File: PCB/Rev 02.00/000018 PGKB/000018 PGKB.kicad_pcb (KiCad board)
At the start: 4 copper layers, 93.5 x 72.5 mm, 154 parts, among them J1 USB Mini B, J2 BM04B-SRSS-TB, U1 SN74HCS365PWR, U2 SN74HCS365PWR, U3 SN74HCS365PWR, U4 W25Q80DVSSIG, U5 RP2040, U6 MCP1825T-3302E/DC, U7 CAT811TTBI-GT3, Y1 12 MHz

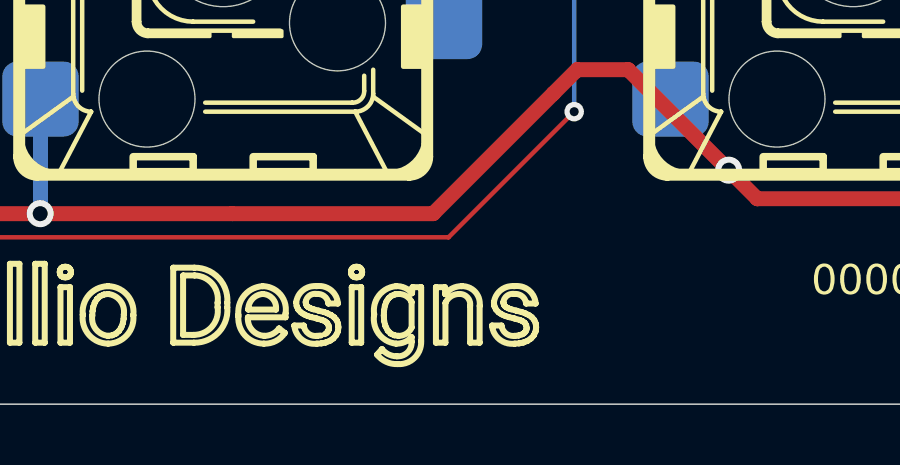
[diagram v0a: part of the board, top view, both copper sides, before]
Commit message: mfg files
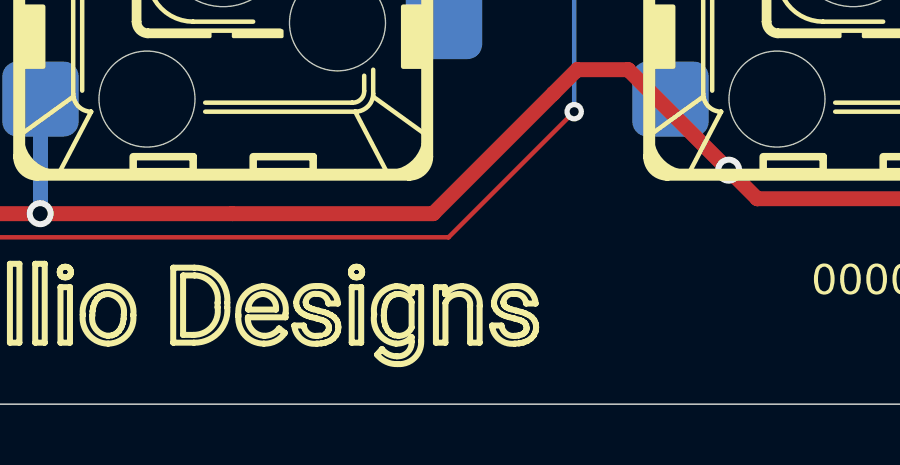
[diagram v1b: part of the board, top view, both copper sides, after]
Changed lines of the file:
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@@
     (fp_arc (start 0.833601 0.096099) (mid 0.973613 -0.257639) (end 1.31605 -0.423381)
       (stroke (width 0.2) (type solid)) (layer "F.SilkS"))
-    (fp_arc (start 1.31605 -0.683114) (mid 1.907699 -0.405492) (end 2.078018 0.225468)
+    (fp_arc (start 1.31605 -0.683114) (mid 1.907695 -0.405492) (end 2.078018 0.225468)
       (stroke (width 0.2) (type solid)) (layer "F.SilkS"))
     (fp_arc (start 1.31605 -0.423379) (mid 1.645394 -0.271037) (end 1.761468 0.072768)
@@
     (fp_arc (start 1.355618 1.232463) (mid 0.731987 0.965619) (end 0.50639 0.325909)
       (stroke (width 0.2) (type solid)) (layer "F.SilkS"))
-    (fp_arc (start 1.372869 0.972724) (mid 0.966364 0.781549) (end 0.82295 0.35584)
+    (fp_arc (start 1.372869 0.972724) (mid 0.966366 0.781547) (end 0.82295 0.35584)
       (stroke (width 0.2) (type solid)) (layer "F.SilkS"))
     (fp_arc (start 1.8609 0.725158) (mid 1.647116 0.90854) (end 1.372868 0.972731)
@@
     (fp_arc (start 3.12764 0.972723) (mid 2.834729 0.892832) (end 2.685781 0.628268)
       (stroke (width 0.2) (type solid)) (layer "F.SilkS"))
-    (fp_arc (start 3.12764 1.232463) (mid 2.619347 1.092399) (end 2.369218 0.628268)
+    (fp_arc (start 3.12764 1.232463) (mid 2.61934 1.092397) (end 2.369218 0.628268)
       (stroke (width 0.2) (type solid)) (layer "F.SilkS"))
-    (fp_arc (start 5.03409 0.259459) (mid 5.19195 -0.37288) (end 5.765118 -0.683118)
+    (fp_arc (start 5.03409 0.259459) (mid 5.191951 -0.372877) (end 5.765118 -0.683118)
       (stroke (width 0.2) (type solid)) (layer "F.SilkS"))
     (fp_arc (start 5.761569 1.232466) (mid 5.184943 0.905126) (end 5.03409 0.259459)
@@
     (fp_arc (start 5.844259 -0.423382) (mid 6.101988 -0.353589) (end 6.28105 -0.155518)
       (stroke (width 0.2) (type solid)) (layer "F.SilkS"))
-    (fp_arc (start 6.280538 1.013814) (mid 6.045436 1.181008) (end 5.761568 1.232468)
+    (fp_arc (start 6.280538 1.013814) (mid 6.045436 1.181019) (end 5.761568 1.232468)
       (stroke (width 0.2) (type solid)) (layer "F.SilkS"))
     (fp_arc (start 6.280541 1.169557) (mid 6.145913 1.523237) (end 5.79099 1.65455)
@@
     (fp_arc (start 7.400665 -0.416784) (mid 7.646446 -0.616044) (end 7.955659 -0.683118)
       (stroke (width 0.2) (type solid)) (layer "F.SilkS"))
-    (fp_arc (start 7.407765 -0.124568) (mid 7.589656 -0.340694) (end 7.859781 -0.423381)
+    (fp_arc (start 7.407765 -0.124568) (mid 7.589655 -0.340729) (end 7.859781 -0.423381)
       (stroke (width 0.2) (type solid)) (layer "F.SilkS"))
     (fp_arc (start 7.859779 -0.42338) (mid 8.138248 -0.314437) (end 8.231131 -0.030218)
       (stroke (width 0.2) (type solid)) (layer "F.SilkS"))
-    (fp_arc (start 7.955657 -0.683113) (mid 8.404847 -0.489303) (end 8.54819 -0.02159)
+    (fp_arc (start 7.955657 -0.683113) (mid 8.404805 -0.489301) (end 8.54819 -0.02159)
       (stroke (width 0.2) (type solid)) (layer "F.SilkS"))
     (fp_arc (start 9.023535 -0.141819) (mid 9.255576 -0.552139) (end 9.7084 -0.683118)
@@
     (fp_arc (start 9.708398 -0.683125) (mid 10.188203 -0.5481) (end 10.415081 -0.104281)
       (stroke (width 0.2) (type solid)) (layer "F.SilkS"))
-    (fp_arc (start 9.708398 -0.423378) (mid 9.96879 -0.344297) (end 10.097 -0.104281)
+    (fp_arc (start 9.708398 -0.423378) (mid 9.968762 -0.344292) (end 10.097 -0.104281)
       (stroke (width 0.2) (type solid)) (layer "F.SilkS"))
     (fp_arc (start 9.71855 0.972726) (mid 9.425639 0.892824) (end 9.276681 0.628268)
       (stroke (width 0.2) (type solid)) (layer "F.SilkS"))
-    (fp_arc (start 9.71855 1.232464) (mid 9.21027 1.092398) (end 8.960131 0.628268)
+    (fp_arc (start 9.71855 1.232464) (mid 9.210242 1.092402) (end 8.960131 0.628268)
       (stroke (width 0.2) (type solid)) (layer "F.SilkS"))
   )

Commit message: MODIFICATIONS To Rev 2
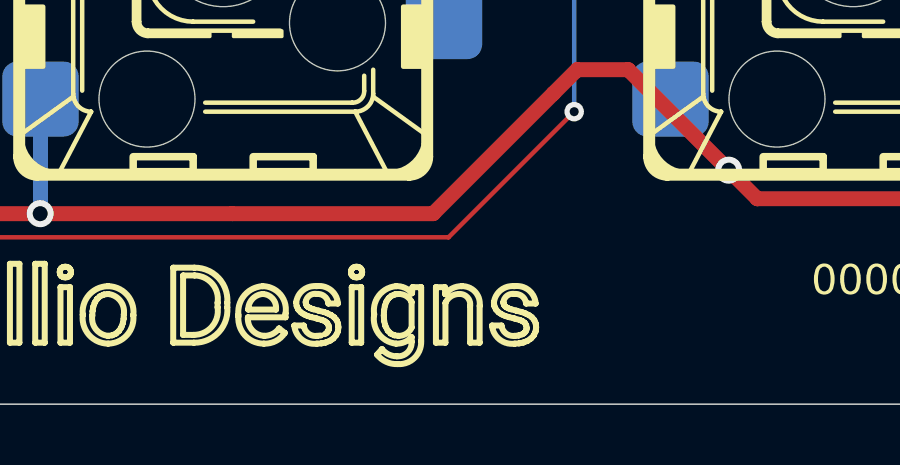
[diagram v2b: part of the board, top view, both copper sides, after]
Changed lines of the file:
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@@
     (fp_arc (start 0.833601 0.096099) (mid 0.973613 -0.257639) (end 1.31605 -0.423381)
       (stroke (width 0.2) (type solid)) (layer "F.SilkS"))
-    (fp_arc (start 1.31605 -0.683114) (mid 1.907695 -0.405492) (end 2.078018 0.225468)
+    (fp_arc (start 1.31605 -0.683114) (mid 1.907699 -0.405492) (end 2.078018 0.225468)
       (stroke (width 0.2) (type solid)) (layer "F.SilkS"))
     (fp_arc (start 1.31605 -0.423379) (mid 1.645394 -0.271037) (end 1.761468 0.072768)
@@
     (fp_arc (start 1.355618 1.232463) (mid 0.731987 0.965619) (end 0.50639 0.325909)
       (stroke (width 0.2) (type solid)) (layer "F.SilkS"))
-    (fp_arc (start 1.372869 0.972724) (mid 0.966366 0.781547) (end 0.82295 0.35584)
+    (fp_arc (start 1.372869 0.972724) (mid 0.966362 0.781547) (end 0.82295 0.35584)
       (stroke (width 0.2) (type solid)) (layer "F.SilkS"))
     (fp_arc (start 1.8609 0.725158) (mid 1.647116 0.90854) (end 1.372868 0.972731)
@@
     (fp_arc (start 3.12764 0.972723) (mid 2.834729 0.892832) (end 2.685781 0.628268)
       (stroke (width 0.2) (type solid)) (layer "F.SilkS"))
-    (fp_arc (start 3.12764 1.232463) (mid 2.61934 1.092397) (end 2.369218 0.628268)
-      (stroke (width 0.2) (type solid)) (layer "F.SilkS"))
-    (fp_arc (start 5.03409 0.259459) (mid 5.191951 -0.372877) (end 5.765118 -0.683118)
+    (fp_arc (start 3.12764 1.232463) (mid 2.619347 1.092399) (end 2.369218 0.628268)
+      (stroke (width 0.2) (type solid)) (layer "F.SilkS"))
+    (fp_arc (start 5.03409 0.259459) (mid 5.19195 -0.37288) (end 5.765118 -0.683118)
       (stroke (width 0.2) (type solid)) (layer "F.SilkS"))
     (fp_arc (start 5.761569 1.232466) (mid 5.184943 0.905126) (end 5.03409 0.259459)
@@
     (fp_arc (start 5.844259 -0.423382) (mid 6.101988 -0.353589) (end 6.28105 -0.155518)
       (stroke (width 0.2) (type solid)) (layer "F.SilkS"))
-    (fp_arc (start 6.280538 1.013814) (mid 6.045436 1.181019) (end 5.761568 1.232468)
+    (fp_arc (start 6.280538 1.013814) (mid 6.045436 1.181008) (end 5.761568 1.232468)
       (stroke (width 0.2) (type solid)) (layer "F.SilkS"))
     (fp_arc (start 6.280541 1.169557) (mid 6.145913 1.523237) (end 5.79099 1.65455)
@@
     (fp_arc (start 7.400665 -0.416784) (mid 7.646446 -0.616044) (end 7.955659 -0.683118)
       (stroke (width 0.2) (type solid)) (layer "F.SilkS"))
-    (fp_arc (start 7.407765 -0.124568) (mid 7.589655 -0.340729) (end 7.859781 -0.423381)
+    (fp_arc (start 7.407765 -0.124568) (mid 7.589656 -0.340694) (end 7.859781 -0.423381)
       (stroke (width 0.2) (type solid)) (layer "F.SilkS"))
     (fp_arc (start 7.859779 -0.42338) (mid 8.138248 -0.314437) (end 8.231131 -0.030218)
       (stroke (width 0.2) (type solid)) (layer "F.SilkS"))
-    (fp_arc (start 7.955657 -0.683113) (mid 8.404805 -0.489301) (end 8.54819 -0.02159)
+    (fp_arc (start 7.955657 -0.683113) (mid 8.404847 -0.489303) (end 8.54819 -0.02159)
       (stroke (width 0.2) (type solid)) (layer "F.SilkS"))
     (fp_arc (start 9.023535 -0.141819) (mid 9.255576 -0.552139) (end 9.7084 -0.683118)
@@
     (fp_arc (start 9.708398 -0.683125) (mid 10.188203 -0.5481) (end 10.415081 -0.104281)
       (stroke (width 0.2) (type solid)) (layer "F.SilkS"))
-    (fp_arc (start 9.708398 -0.423378) (mid 9.968762 -0.344292) (end 10.097 -0.104281)
+    (fp_arc (start 9.708398 -0.423378) (mid 9.96879 -0.344297) (end 10.097 -0.104281)
       (stroke (width 0.2) (type solid)) (layer "F.SilkS"))
     (fp_arc (start 9.71855 0.972726) (mid 9.425639 0.892824) (end 9.276681 0.628268)
       (stroke (width 0.2) (type solid)) (layer "F.SilkS"))
-    (fp_arc (start 9.71855 1.232464) (mid 9.210242 1.092402) (end 8.960131 0.628268)
+    (fp_arc (start 9.71855 1.232464) (mid 9.21027 1.092398) (end 8.960131 0.628268)
       (stroke (width 0.2) (type solid)) (layer "F.SilkS"))
   )
@@
         (effects (font (size 0.8 0.8) (thickness 0.15)) (justify bottom))
     )
-    (fp_text value "4954" (at 0 0 -180) (layer "F.Fab") hide
+    (fp_text value "4954" (at 0 0) (layer "F.Fab") hide
         (effects (font (size 0.8 0.8) (thickness 0.15)))
     )
-    (fp_text user "${REFERENCE}" (at 0 0 -90) (layer "F.Fab")
+    (fp_text user "${REFERENCE}" (at 0 0 90) (layer "F.Fab")
         (effects (font (size 0.44 0.44) (thickness 0.06)))
     )

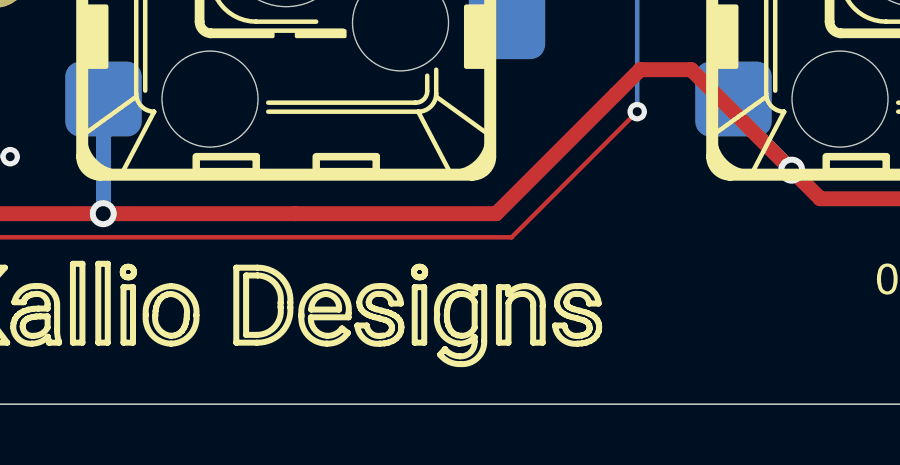
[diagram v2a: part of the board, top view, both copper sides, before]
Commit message: MODIFICATIONS Updates
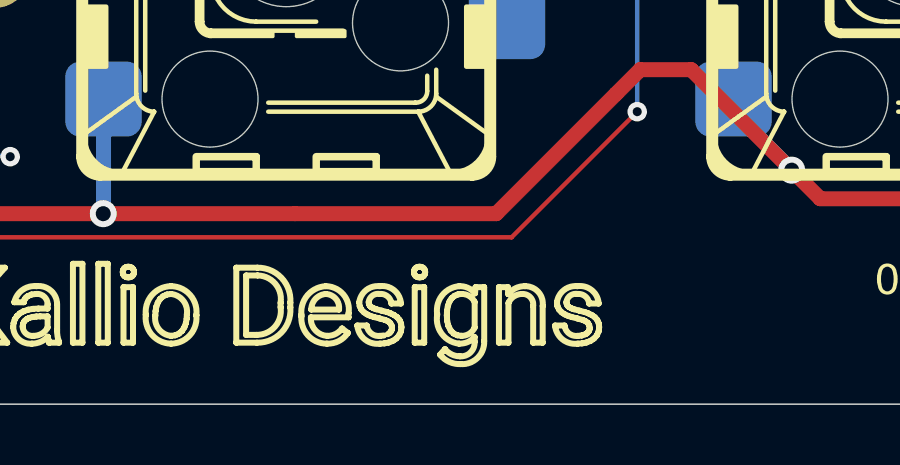
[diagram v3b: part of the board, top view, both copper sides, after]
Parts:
- J1: value USB Mini B -> USB C
- S20: value symbol_template -> PEC11R-4215K-S0012
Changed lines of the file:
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@@
     (fp_arc (start 0.833601 0.096099) (mid 0.973613 -0.257639) (end 1.31605 -0.423381)
       (stroke (width 0.2) (type solid)) (layer "F.SilkS"))
-    (fp_arc (start 1.31605 -0.683114) (mid 1.907699 -0.405492) (end 2.078018 0.225468)
+    (fp_arc (start 1.31605 -0.683114) (mid 1.907695 -0.405492) (end 2.078018 0.225468)
       (stroke (width 0.2) (type solid)) (layer "F.SilkS"))
     (fp_arc (start 1.31605 -0.423379) (mid 1.645394 -0.271037) (end 1.761468 0.072768)
@@
     (fp_arc (start 1.355618 1.232463) (mid 0.731987 0.965619) (end 0.50639 0.325909)
       (stroke (width 0.2) (type solid)) (layer "F.SilkS"))
-    (fp_arc (start 1.372869 0.972724) (mid 0.966362 0.781547) (end 0.82295 0.35584)
+    (fp_arc (start 1.372869 0.972724) (mid 0.96636 0.78155) (end 0.82295 0.35584)
       (stroke (width 0.2) (type solid)) (layer "F.SilkS"))
     (fp_arc (start 1.8609 0.725158) (mid 1.647116 0.90854) (end 1.372868 0.972731)
@@
     (fp_arc (start 3.12764 0.972723) (mid 2.834729 0.892832) (end 2.685781 0.628268)
       (stroke (width 0.2) (type solid)) (layer "F.SilkS"))
-    (fp_arc (start 3.12764 1.232463) (mid 2.619347 1.092399) (end 2.369218 0.628268)
+    (fp_arc (start 3.12764 1.232463) (mid 2.61934 1.092397) (end 2.369218 0.628268)
       (stroke (width 0.2) (type solid)) (layer "F.SilkS"))
-    (fp_arc (start 5.03409 0.259459) (mid 5.19195 -0.37288) (end 5.765118 -0.683118)
+    (fp_arc (start 5.03409 0.259459) (mid 5.191951 -0.372877) (end 5.765118 -0.683118)
       (stroke (width 0.2) (type solid)) (layer "F.SilkS"))
     (fp_arc (start 5.761569 1.232466) (mid 5.184943 0.905126) (end 5.03409 0.259459)
@@
     (fp_arc (start 5.844259 -0.423382) (mid 6.101988 -0.353589) (end 6.28105 -0.155518)
       (stroke (width 0.2) (type solid)) (layer "F.SilkS"))
-    (fp_arc (start 6.280538 1.013814) (mid 6.045436 1.181008) (end 5.761568 1.232468)
+    (fp_arc (start 6.280538 1.013814) (mid 6.045436 1.181019) (end 5.761568 1.232468)
       (stroke (width 0.2) (type solid)) (layer "F.SilkS"))
     (fp_arc (start 6.280541 1.169557) (mid 6.145913 1.523237) (end 5.79099 1.65455)
@@
     (fp_arc (start 7.400665 -0.416784) (mid 7.646446 -0.616044) (end 7.955659 -0.683118)
       (stroke (width 0.2) (type solid)) (layer "F.SilkS"))
-    (fp_arc (start 7.407765 -0.124568) (mid 7.589656 -0.340694) (end 7.859781 -0.423381)
+    (fp_arc (start 7.407765 -0.124568) (mid 7.589655 -0.340729) (end 7.859781 -0.423381)
       (stroke (width 0.2) (type solid)) (layer "F.SilkS"))
     (fp_arc (start 7.859779 -0.42338) (mid 8.138248 -0.314437) (end 8.231131 -0.030218)
       (stroke (width 0.2) (type solid)) (layer "F.SilkS"))
-    (fp_arc (start 7.955657 -0.683113) (mid 8.404847 -0.489303) (end 8.54819 -0.02159)
+    (fp_arc (start 7.955657 -0.683113) (mid 8.404805 -0.489301) (end 8.54819 -0.02159)
       (stroke (width 0.2) (type solid)) (layer "F.SilkS"))
     (fp_arc (start 9.023535 -0.141819) (mid 9.255576 -0.552139) (end 9.7084 -0.683118)
@@
     (fp_arc (start 9.708398 -0.683125) (mid 10.188203 -0.5481) (end 10.415081 -0.104281)
       (stroke (width 0.2) (type solid)) (layer "F.SilkS"))
-    (fp_arc (start 9.708398 -0.423378) (mid 9.96879 -0.344297) (end 10.097 -0.104281)
+    (fp_arc (start 9.708398 -0.423378) (mid 9.968762 -0.344292) (end 10.097 -0.104281)
       (stroke (width 0.2) (type solid)) (layer "F.SilkS"))
     (fp_arc (start 9.71855 0.972726) (mid 9.425639 0.892824) (end 9.276681 0.628268)
       (stroke (width 0.2) (type solid)) (layer "F.SilkS"))
-    (fp_arc (start 9.71855 1.232464) (mid 9.21027 1.092398) (end 8.960131 0.628268)
+    (fp_arc (start 9.71855 1.232464) (mid 9.210242 1.092402) (end 8.960131 0.628268)
       (stroke (width 0.2) (type solid)) (layer "F.SilkS"))
   )
@@
     (at 120.9 118.45)
     (tags "rotary encoder")
-    (property "Code" "PEC11R-4215K-S0012")
     (property "DNP" "F")
     (property "MFG_PartNo" "PEC11R-4215K-S0012")
@@
         (effects (font (size 0.8 0.8) (thickness 0.15)))
     )
-    (fp_text value "symbol_template" (at 9.1 0.2 90) (layer "F.Fab") hide
+    (fp_text value "PEC11R-4215K-S0012" (at 9.1 0.2 90) (layer "F.Fab") hide
         (effects (font (size 0.8 0.8) (thickness 0.15)))
     )
@@
     (tags "USB Type-C Receptacle Through-hole Right angle")
     (property "DNP" "F")
-    (property "MFG_PartNo" "USB-B-S-VT")
-    (property "Manufacturer" "Adam Tech")
-    (property "Price" "1")
+    (property "MFG_PartNo" "USB4085-GF-A")
+    (property "Manufacturer" "GCT")
+    (property "Price" "0.85")
     (property "Sheetfile" "USBcon.kicad_sch")
     (property "Sheetname" "USB Connector")
     (property "Supplier" "Digi-Key")
-    (property "Supplier_PartNo" "2057-USB-B-S-VT-ND")
-    (property "ki_description" "USB Mini Vertical Connector")
-    (property "ki_keywords" "USB Mini Vertical Connector")
+    (property "Supplier_PartNo" "2073-USB4085-GF-ACT-ND")
+    (property "ki_description" "CONN RCPT USB2.0 TYPE C 16+8POS")
+    (property "ki_keywords" "CONN RCPT USB2.0 TYPE C 16+8POS")
     (attr through_hole)
     (fp_text reference "J1" (at 2.975 1.8) (layer "B.SilkS")
         (effects (font (size 0.8 0.8) (thickness 0.15)) (justify mirror))
     )
-    (fp_text value "USB Mini B" (at 2.975 -9.925) (layer "B.Fab") hide
+    (fp_text value "USB C" (at 2.975 -9.925) (layer "B.Fab") hide
         (effects (font (size 0.8 0.8) (thickness 0.15)) (justify mirror))
     )
